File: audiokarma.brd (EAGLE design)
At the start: 162.2 x 102.9 mm, 63 parts, among them IC1 OPA2134U, IC2 OPA2134U

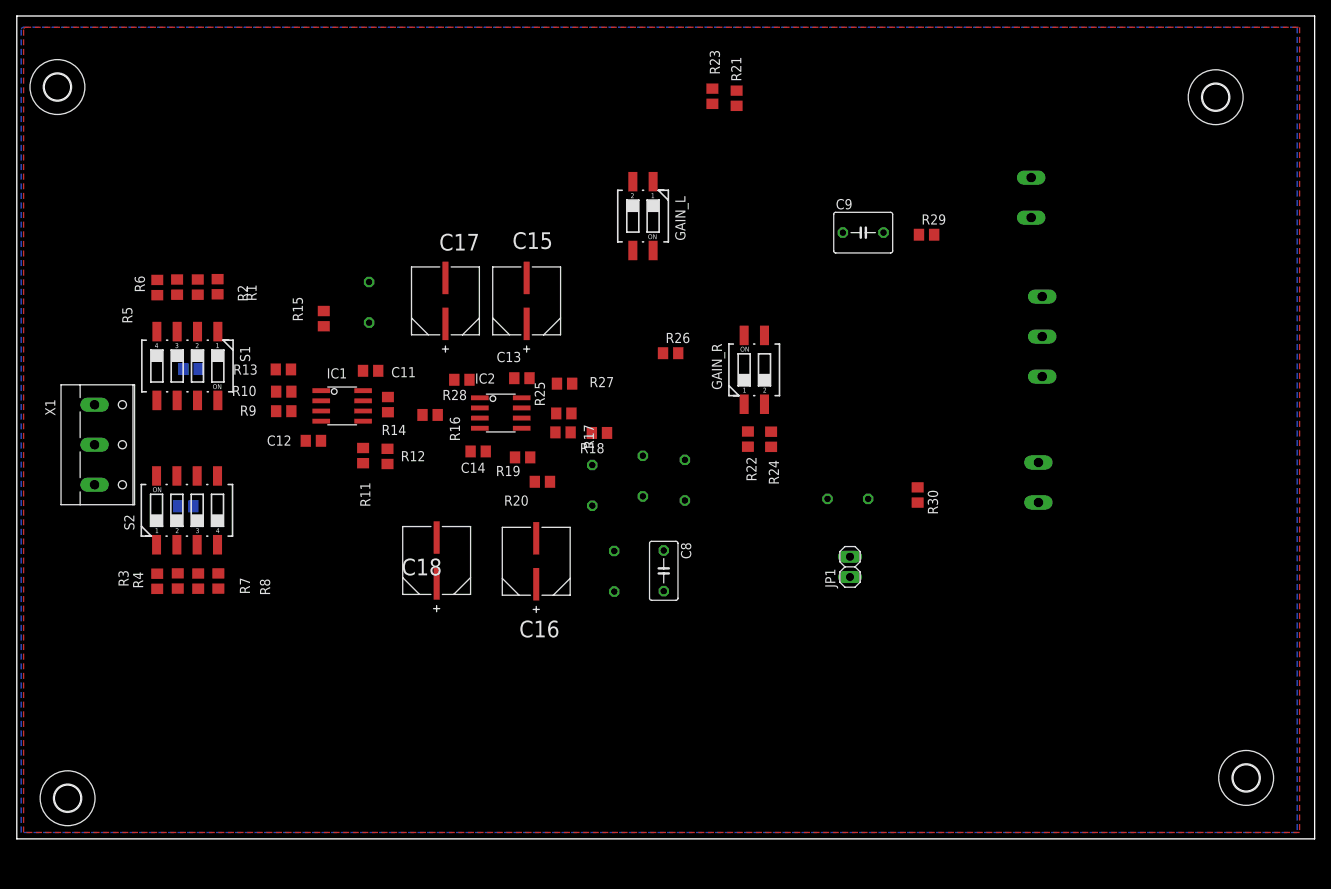
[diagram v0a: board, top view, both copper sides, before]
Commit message: colocados al 90%
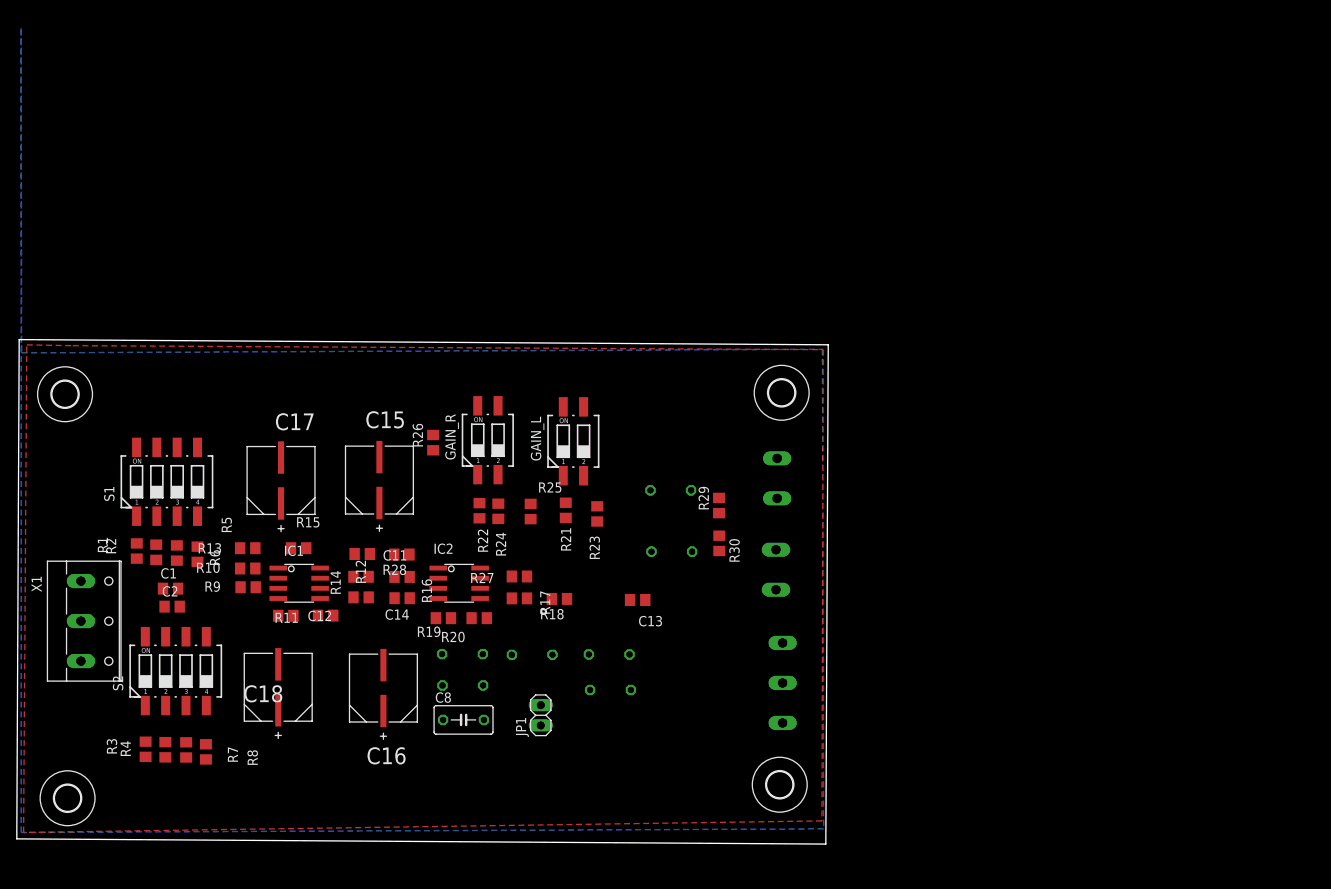
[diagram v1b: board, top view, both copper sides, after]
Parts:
- moved H2 65.6 mm to (95.6, 55.8)
- moved H4 58.3 mm to (95.4, 6.77)
- moved R21 55.8 mm to (68.6, 41.1), turned to 90 degrees
- moved R23 54.2 mm to (72.5, 40.6), turned to 90 degrees
- moved X4 54.1 mm to (94.4, 19.5)
- moved C3 48.5 mm to (64.4, 23.0), turned to 180 degrees
- moved X2 47.3 mm to (96.3, 45.1)
- moved JP1 42.9 mm to (65.5, 15.4)
- moved R29 42.6 mm to (87.8, 41.7), turned to 90 degrees
- moved C9 40.2 mm to (81.8, 43.6), flipped to the bottom, turned to 180 degrees
- moved H1 38.4 mm to (6.03, 55.6)
- moved R24 35.3 mm to (60.2, 41.0)
- moved R22 34.7 mm to (57.8, 41.0)
- moved X3 34.6 mm to (96.2, 33.6)
- moved R1 34.5 mm to (15.0, 36.0), turned to 90 degrees
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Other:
- board size 162.2 x 102.9 mm -> 101.4 x 63.1 mm

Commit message: 95
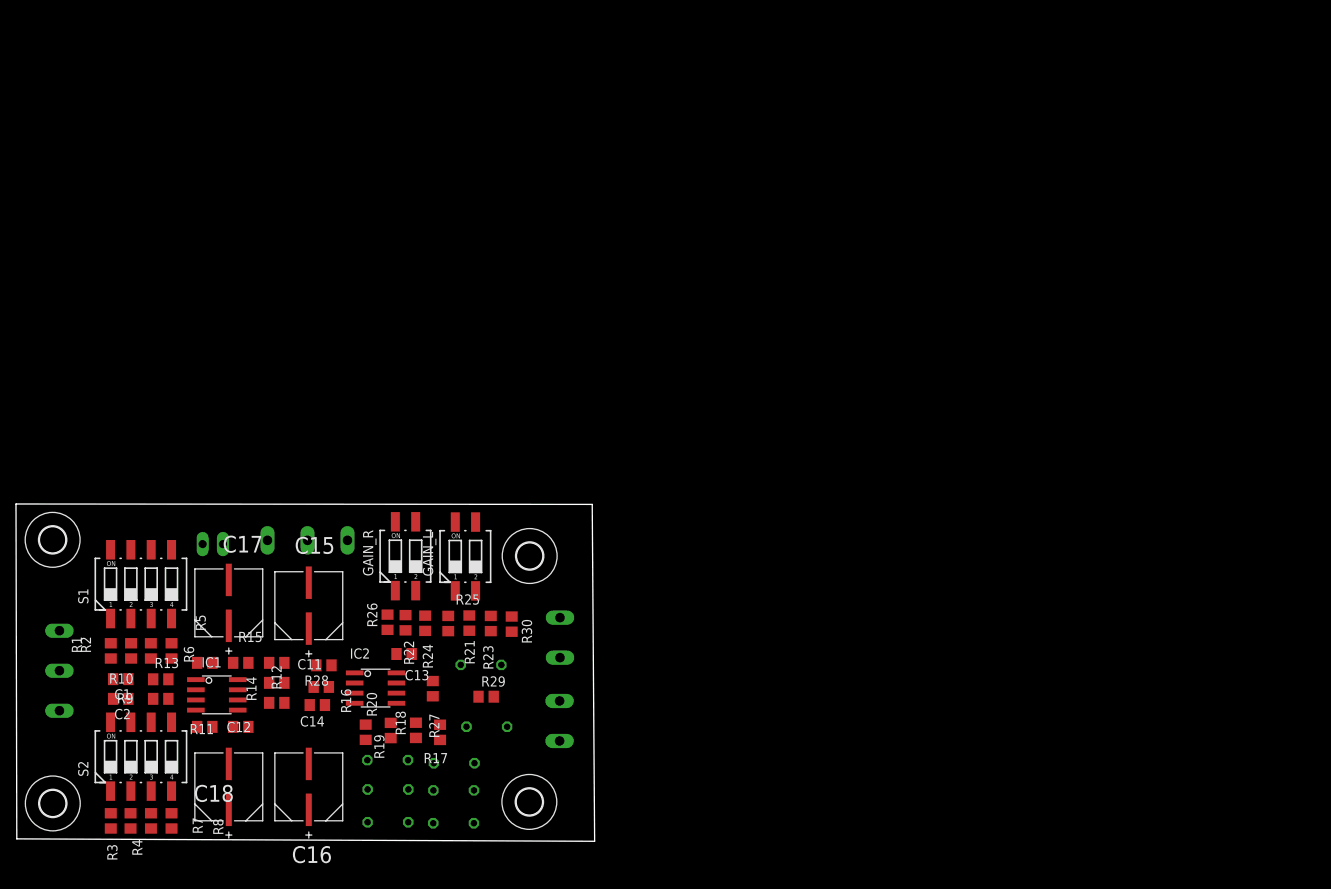
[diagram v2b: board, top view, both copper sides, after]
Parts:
- moved X4 61.2 mm to (36.3, 38.6), turned to 0 degrees
- moved JP1 46.2 mm to (24.5, 36.9), flipped to the bottom, turned to 0 degrees
- moved X2 42.5 mm to (66.6, 14.7), turned to 270 degrees
- moved R29 37.7 mm to (58.7, 17.8), turned to 0 degrees
- moved H2 37.5 mm to (64.1, 35.4)
- moved C9 37.4 mm to (58.8, 14.0)
- moved H4 31.4 mm to (64.1, 4.62)
- moved X3 30.7 mm to (66.6, 25.1), turned to 270 degrees
- moved C13 30.0 mm to (48.4, 23.1)
- moved C5 28.7 mm to (54.6, 1.96)
- moved R30 27.8 mm to (61.9, 26.8)
- moved C10 27.7 mm to (58.0, 21.8)
- moved R18 24.3 mm to (49.9, 13.6), turned to 90 degrees
- moved C7 23.3 mm to (54.6, 6.06)
- moved R26 23.2 mm to (46.3, 27.1)
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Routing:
- removed copper zone on layer 1, net AGND
- removed copper zone on layer 16, net AGND
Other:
- board size 101.4 x 63.1 mm -> 72.3 x 42.2 mm
